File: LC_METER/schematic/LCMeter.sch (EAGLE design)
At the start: 208 parts, among them IC1 MEGA8535, IC10 MC34063, IC2 74HC595, IC3 74HC595, IC4 74HC595, IC5 74HC595, IC6 74HC595, IC7 LM324, IC8 7905, IC9 LM317, J10 0, J11 0, J4 0, J6 0, J8 0, J9 0, Q1 12MHz, T1 BC847, T2 BC857, T3 BC847, T4 BC847, T5 BC847, T6 BC847, T7 BC857, X1 MCU_PROGRAMMING, X2 L_X, X3 C_X, X4 USB_MICRO, X5 USB_B

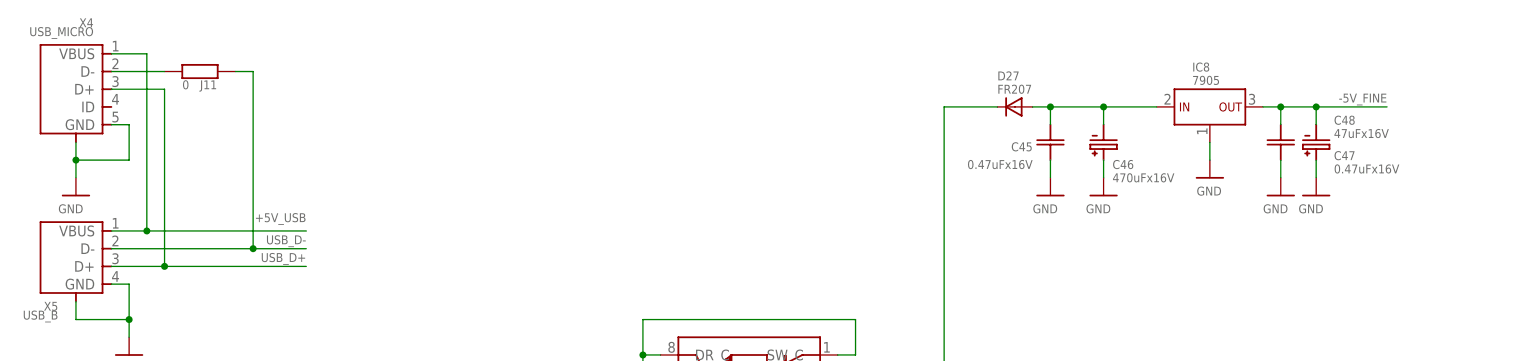
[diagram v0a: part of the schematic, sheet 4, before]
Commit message: LCMeter start routing2
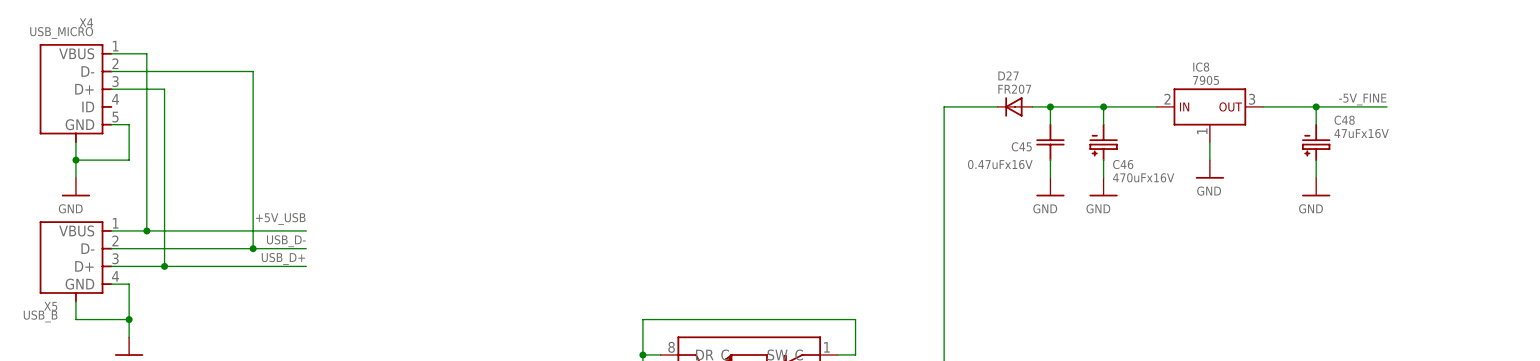
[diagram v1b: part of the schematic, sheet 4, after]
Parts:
- removed C47: 0.47uFx16V, __MyCommonLib1:CSMD_0805
- removed J11, J9: 0, __MyCommonLib1:RSMD_0805
- D29: device __MyCommonLib1:1N4001DO-41_10MM -> __MyCommonLib1:1N4001DO-41_5MM
- R81, R82: device __MyCommonLib1:RSMD_1206_BIG_GAP -> __MyCommonLib1:RSMD_0805
- R84: device __MyCommonLib1:RSMD_0805 -> __MyCommonLib1:R0207
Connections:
- removed net N$104: IC6.SER_CLK, J9.PIN1
- removed net N$132: J11.PIN1, X4.D-
- net -5V_FINE: no longer C47.PIN1
- net GND: no longer C47.PIN0
- net LED_SCK': now also IC6.SER_CLK; no longer J9.PIN0
- net USB_D-: now also X4.D-; no longer J11.PIN0
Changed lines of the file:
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@@
 <part name="J6" library="__MyCommonLib1" deviceset="R" device="SMD_0805" value="0"/>
 <part name="J8" library="__MyCommonLib1" deviceset="R" device="SMD_0805" value="0"/>
-<part name="J9" library="__MyCommonLib1" deviceset="R" device="SMD_0805" value="0"/>
 <part name="J10" library="__MyCommonLib1" deviceset="R" device="SMD_0805" value="0"/>
 <part name="C10" library="__MyCommonLib1" deviceset="C" device="SMD_0805" value="0.1uF"/>
@@
 <part name="X4" library="__MyCommonLib1" deviceset="USB_MICRO" device="MICRO" value="USB_MICRO"/>
 <part name="GND70" library="supply1" deviceset="GND" device=""/>
-<part name="J11" library="__MyCommonLib1" deviceset="R" device="SMD_0805" value="0"/>
 <part name="IC10" library="__MyCommonLib1" deviceset="MC34063" device="(SO-8)" value="MC34063"/>
 <part name="TR1" library="__MyCommonLib1" deviceset="TRANS_3WIND" device="RING25X10_HOR" value="TRANS"/>
@@
 <part name="GND72" library="supply1" deviceset="GND" device=""/>
 <part name="D28" library="__MyCommonLib1" deviceset="1N4001" device="DO-41_10MM" value="FR207"/>
-<part name="D29" library="__MyCommonLib1" deviceset="1N4001" device="DO-41_10MM" value="FR207"/>
+<part name="D29" library="__MyCommonLib1" deviceset="1N4001" device="DO-41_5MM" value="FR207"/>
 <part name="C56" library="__MyCommonLib1" deviceset="C" device="SMD_1206_BIG_GAP" value="0.47uFx16V"/>
 <part name="C57" library="__MyCommonLib1" deviceset="CE" device="10MM" value="470uFx16V"/>
 <part name="GND73" library="supply1" deviceset="GND" device=""/>
 <part name="GND74" library="supply1" deviceset="GND" device=""/>
-<part name="R84" library="__MyCommonLib1" deviceset="R" device="SMD_0805" value="5K1"/>
+<part name="R84" library="__MyCommonLib1" deviceset="R" device="0207" value="5K1"/>
 <part name="R85" library="__MyCommonLib1" deviceset="R" device="SMD_0805" value="1K7"/>
 <part name="GND75" library="supply1" deviceset="GND" device=""/>
@@
 <part name="GND79" library="supply1" deviceset="GND" device=""/>
 <part name="GND80" library="supply1" deviceset="GND" device=""/>
-<part name="R81" library="__MyCommonLib1" deviceset="R" device="SMD_1206_BIG_GAP" value="5K1"/>
-<part name="R82" library="__MyCommonLib1" deviceset="R" device="SMD_1206_BIG_GAP" value="1K7"/>
+<part name="R81" library="__MyCommonLib1" deviceset="R" device="SMD_0805" value="5K1"/>
+<part name="R82" library="__MyCommonLib1" deviceset="R" device="SMD_0805" value="1K7"/>
 <part name="IC8" library="__MyCommonLib1" deviceset="7905" device="(D2PAK)" value="7905"/>
-<part name="C47" library="__MyCommonLib1" deviceset="C" device="SMD_0805" value="0.47uFx16V"/>
-<part name="GND81" library="supply1" deviceset="GND" device=""/>
 <part name="GND82" library="supply1" deviceset="GND" device=""/>
 <part name="GND83" library="supply1" deviceset="GND" device=""/>
@@
 <attribute name="VALUE" x="58.42" y="60.96" size="1.27" layer="96" font="vector" ratio="20" rot="MR180"/>
 </instance>
-<instance part="J9" gate="R$1" x="55.88" y="33.02" smashed="yes" rot="MR90">
-<attribute name="NAME" x="50.8" y="35.56" size="1.27" layer="95" font="vector" ratio="20" rot="MR180"/>
-<attribute name="VALUE" x="58.42" y="35.56" size="1.27" layer="96" font="vector" ratio="20" rot="MR180"/>
-</instance>
 <instance part="J10" gate="R$1" x="55.88" y="25.4" smashed="yes" rot="MR90">
 <attribute name="NAME" x="50.8" y="27.94" size="1.27" layer="95" font="vector" ratio="20" rot="MR180"/>
@@
 <junction x="45.72" y="149.86"/>
 <junction x="45.72" y="132.08"/>
-<pinref part="J9" gate="R$1" pin="PIN0"/>
-<wire x1="50.8" y1="33.02" x2="45.72" y2="33.02" width="0.1524" layer="91"/>
 <junction x="45.72" y="66.04"/>
 <junction x="45.72" y="99.06"/>
@@
 <pinref part="IC5" gate="G$1" pin="SER_CLK"/>
 <wire x1="68.58" y1="66.04" x2="45.72" y2="66.04" width="0.1524" layer="91"/>
+<pinref part="IC6" gate="G$1" pin="SER_CLK"/>
+<wire x1="45.72" y1="33.02" x2="68.58" y2="33.02" width="0.1524" layer="91"/>
 </segment>
 </net>
@@
 </segment>
 </net>
-<net name="N$104" class="0">
-<segment>
-<pinref part="IC6" gate="G$1" pin="SER_CLK"/>
-<pinref part="J9" gate="R$1" pin="PIN1"/>
-<wire x1="60.96" y1="33.02" x2="68.58" y2="33.02" width="0.1524" layer="91"/>
-</segment>
-</net>
 <net name="N$107" class="0">
 <segment>
@@
 <attribute name="VALUE" x="17.78" y="134.62" size="1.27" layer="96" font="vector" ratio="20"/>
 </instance>
-<instance part="J11" gate="R$1" x="38.1" y="154.94" smashed="yes" rot="R90">
-<attribute name="NAME" x="38.1" y="152.4" size="1.27" layer="95" font="vector" ratio="20"/>
-<attribute name="VALUE" x="35.56" y="152.4" size="1.27" layer="96" font="vector" ratio="20"/>
-</instance>
 <instance part="IC10" gate="G$1" x="116.84" y="106.68" smashed="yes">
 <attribute name="NAME" x="111.76" y="93.98" size="1.27" layer="95" font="vector" ratio="20" rot="R180"/>
@@
 <attribute name="VALUE" x="180.34" y="153.035" size="1.27" layer="96" font="vector" ratio="20"/>
 </instance>
-<instance part="C47" gate="C$1" x="193.04" y="144.78" smashed="yes">
-<attribute name="NAME" x="200.66" y="142.24" size="1.27" layer="95" font="vector" ratio="20"/>
-<attribute name="VALUE" x="200.66" y="140.335" size="1.27" layer="96" font="vector" ratio="20"/>
-</instance>
-<instance part="GND81" gate="1" x="193.04" y="137.16" smashed="yes">
-<attribute name="VALUE" x="190.5" y="134.62" size="1.27" layer="96" font="vector" ratio="20"/>
-</instance>
 <instance part="GND82" gate="1" x="198.12" y="137.16" smashed="yes">
 <attribute name="VALUE" x="195.58" y="134.62" size="1.27" layer="96" font="vector" ratio="20"/>
@@
 </segment>
 <segment>
-<pinref part="C47" gate="C$1" pin="PIN0"/>
-<pinref part="GND81" gate="1" pin="GND"/>
-<wire x1="193.04" y1="142.24" x2="193.04" y2="139.7" width="0.1524" layer="91"/>
-</segment>
-<segment>
 <pinref part="IC8" gate="G$1" pin="GND"/>
 <pinref part="GND83" gate="1" pin="GND"/>
@@
 <junction x="45.72" y="129.54"/>
 <label x="53.34" y="131.445" size="1.27" layer="95" font="vector" ratio="20" rot="R180"/>
-<pinref part="J11" gate="R$1" pin="PIN0"/>
-<wire x1="43.18" y1="154.94" x2="45.72" y2="154.94" width="0.1524" layer="91"/>
 <wire x1="45.72" y1="154.94" x2="45.72" y2="129.54" width="0.1524" layer="91"/>
+<pinref part="X4" gate="X$1" pin="D-"/>
+<wire x1="25.4" y1="154.94" x2="45.72" y2="154.94" width="0.1524" layer="91"/>
 </segment>
 </net>
@@
 </segment>
 </net>
-<net name="N$132" class="0">
-<segment>
-<pinref part="X4" gate="X$1" pin="D-"/>
-<pinref part="J11" gate="R$1" pin="PIN1"/>
-<wire x1="33.02" y1="154.94" x2="25.4" y2="154.94" width="0.1524" layer="91"/>
-</segment>
-</net>
 <net name="N$10" class="0">
 <segment>
@@
 <segment>
 <pinref part="IC8" gate="G$1" pin="OUT"/>
-<wire x1="190.5" y1="149.86" x2="193.04" y2="149.86" width="0.1524" layer="91"/>
-<pinref part="C47" gate="C$1" pin="PIN1"/>
-<wire x1="193.04" y1="147.32" x2="193.04" y2="149.86" width="0.1524" layer="91"/>
-<junction x="193.04" y="149.86"/>
-<wire x1="193.04" y1="149.86" x2="198.12" y2="149.86" width="0.1524" layer="91"/>
+<wire x1="190.5" y1="149.86" x2="198.12" y2="149.86" width="0.1524" layer="91"/>
 <label x="208.28" y="151.765" size="1.27" layer="95" font="vector" ratio="20" rot="R180"/>
 <pinref part="C48" gate="C$1" pin="-"/>
